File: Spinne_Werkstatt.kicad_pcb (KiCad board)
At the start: 2 copper layers, 15 parts, among them J1 Conn_01x02_Pin, J3 Conn_01x03_Pin, Q1 BSS138, Q2 BSS138, U2 CH340C, U4 ESP32-WROOM-32

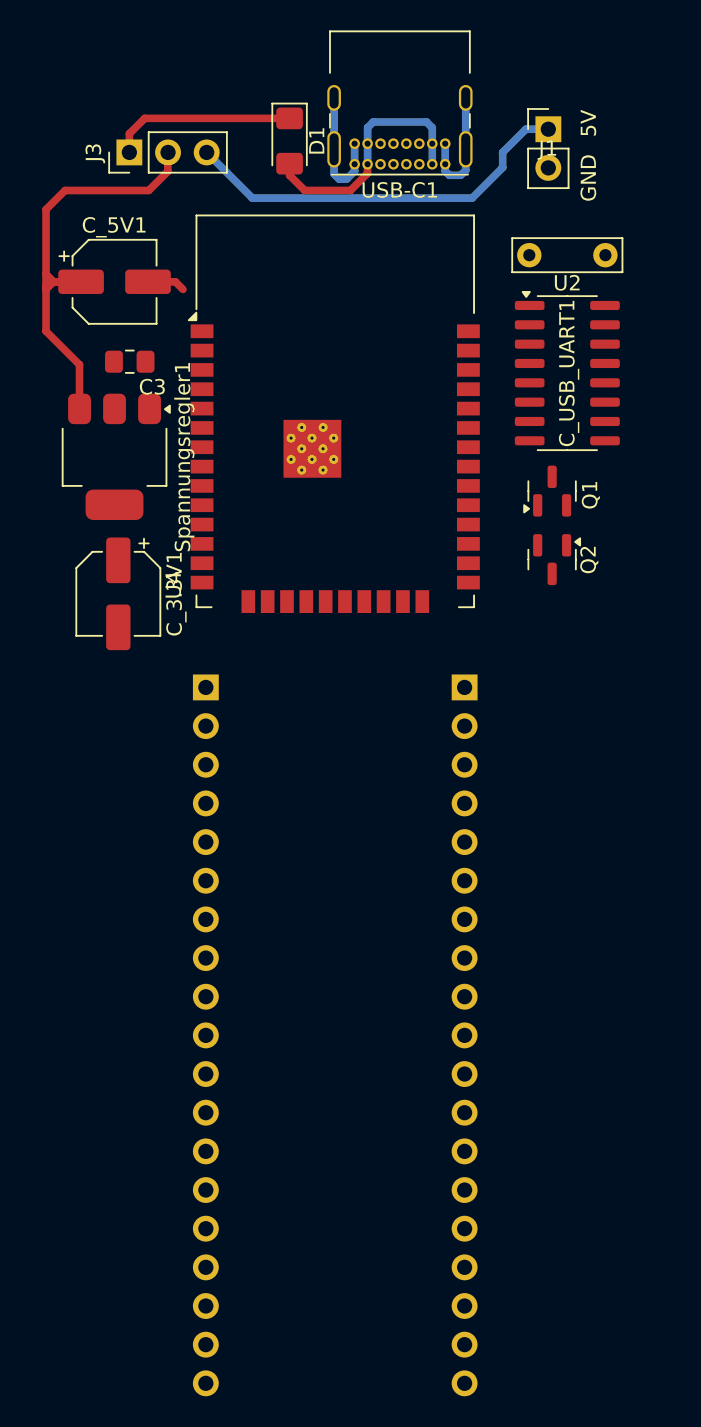
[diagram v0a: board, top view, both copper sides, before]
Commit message: finished first pcb -- ugly
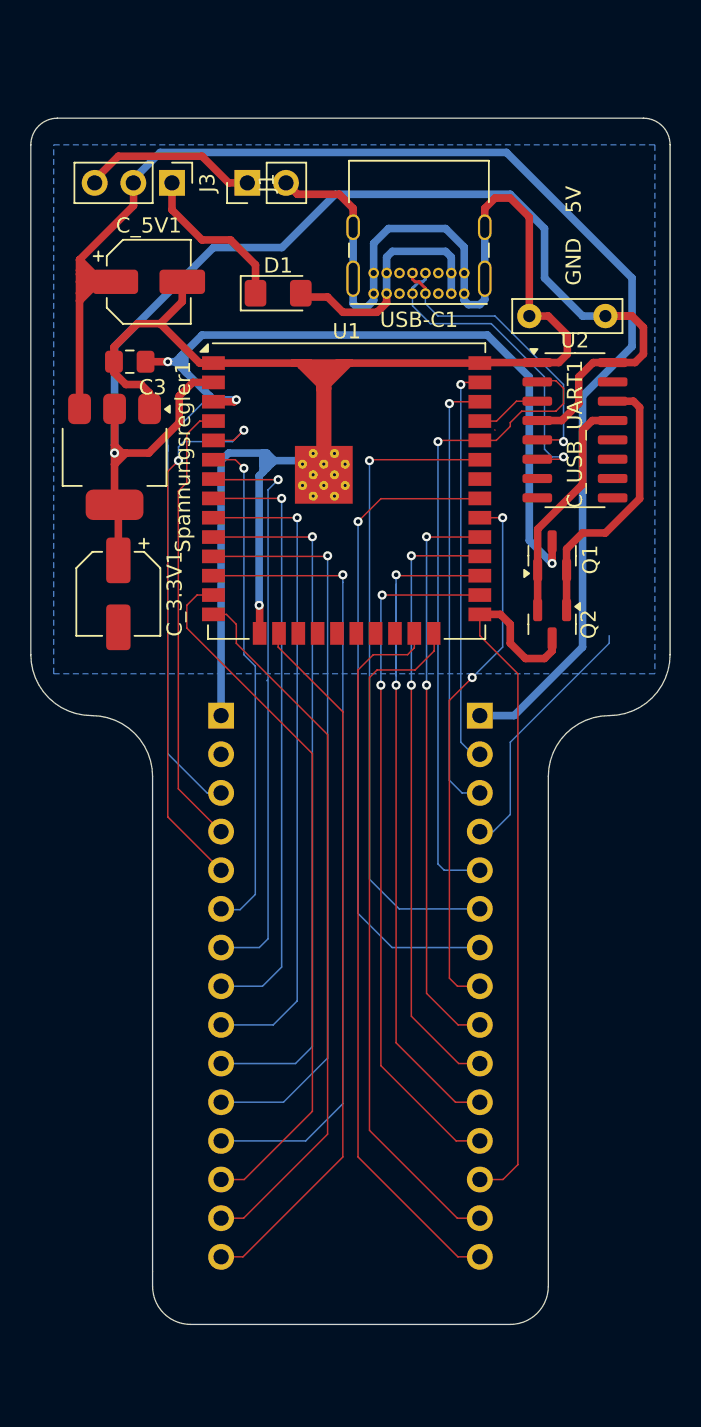
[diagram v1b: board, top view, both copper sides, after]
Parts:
- removed U4: ESP32-WROOM-32, bulme_footprints:ESP32-WROOM-32D
- added U1: ESP32-WROOM-32UE, RF_Module:ESP32-WROOM-32UE, F.Cu at (139.2, 62.8)
- esp_left1, esp_right1: value Conn_01x19_Pin -> Conn_01x15_Pin; footprint Connector_PinHeader_2.54mm:PinHeader_1x19_P2.54mm_Vertical -> Connector_PinHeader_2.54mm:PinHeader_1x15_P2.54mm_Vertical
- moved J1 20.1 mm to (132.7, 42.5), turned to 90 degrees
- moved D1 10.0 mm to (134.8, 49.8), turned to 0 degrees
- moved USB-C1 8.59 mm to (147.0, 49.8)
- moved Q1 4.25 mm to (152.8, 67.0)
- moved Q2 4.25 mm to (152.8, 71.5)
- moved C_USB_UART1 4.00 mm to (156.2, 51.2)
- moved U2 3.78 mm to (154.2, 58.8)
- moved J3 3.44 mm to (127.8, 42.5), turned to -90 degrees
- moved C_5V1 2.25 mm to (126.2, 49.0)
- moved esp_left1 2.10 mm to (131.0, 77.5)
- moved esp_right1 2.10 mm to (148.0, 77.5)
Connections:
- esp_left1 pad 15: pin15 -> pin16
- esp_right1 pad 10: pin29 -> pin28
- esp_right1 pad 11: pin28 -> pin27
- esp_right1 pad 12: pin27 -> pin26
- esp_right1 pad 13: pin26 -> ESP32_IO0
- esp_right1 pad 14: pin25 -> pin24
- esp_right1 pad 15: pin24 -> pin23
- esp_right1 pad 2: GND -> pin37
- esp_right1 pad 3: pin37 -> pin36
- esp_right1 pad 4: pin36 -> ESP32_TX
- esp_right1 pad 5: ESP32_TX -> ESP32_RX
- esp_right1 pad 6: ESP32_RX -> pin33
- esp_right1 pad 7: pin33 -> pin31
- esp_right1 pad 8: pin31 -> pin30
- esp_right1 pad 9: pin30 -> pin29
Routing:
- net GND: track 19.5 -> 164.2 mm, vias 0 -> 1
- net +3V3: track 0.00 -> 86.5 mm, vias 0 -> 1
- net ESP32_EN: track 0.00 -> 80.3 mm, vias 0 -> 3
- net +5V: track 30.1 -> 99.3 mm
- net pin12: track 0.00 -> 52.1 mm, vias 0 -> 1
- net pin27: track 0.00 -> 49.7 mm, vias 0 -> 2
- net pin23: track 0.00 -> 48.7 mm
- net pin11: track 0.00 -> 48.7 mm, vias 0 -> 1
- net ESP32_IO0: track 0.00 -> 47.8 mm
- net pin14: track 0.00 -> 47.0 mm
- net pin16: track 0.00 -> 46.9 mm
- net pin13: track 0.00 -> 46.6 mm
- net pin10: track 0.00 -> 46.5 mm, vias 0 -> 1
- net pin26: track 0.00 -> 46.0 mm, vias 0 -> 2
- net pin24: track 0.00 -> 45.6 mm
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- added copper zone on B.Cu, net GND
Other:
- board outline added: 42 x 79.2 mm

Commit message: nearly finished, not perfect but ok
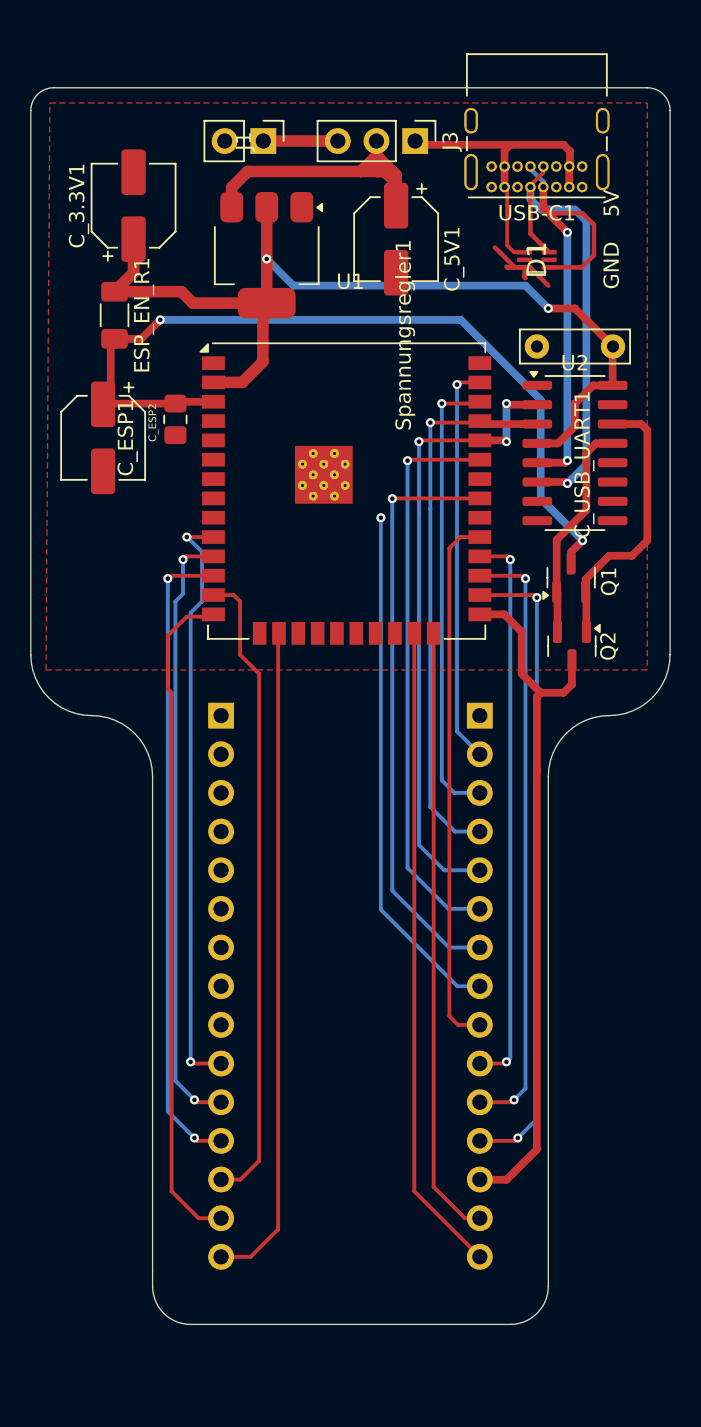
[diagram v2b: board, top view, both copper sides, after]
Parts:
- removed C3: 1uF, Capacitor_SMD:C_0805_2012Metric_Pad1.18x1.45mm_HandSolder
- added C_ESP1: 22uF, Capacitor_SMD:CP_Elec_5x5.7, F.Cu at (123.2, 59.2)
- added C_ESP2: 100nF, Capacitor_SMD:C_0805_2012Metric_Pad1.18x1.45mm_HandSolder, F.Cu at (128.0, 58.0)
- added ESP_EN_R1: 10k, Resistor_SMD:R_1206_3216Metric_Pad1.30x1.75mm_HandSolder, F.Cu at (124.0, 51.2)
- D1: value D_Schottky -> ESDAULC6-3BP6; footprint Diode_SMD:D_1206_3216Metric_Pad1.42x1.75mm_HandSolder -> bulme_footprints:ESDAULC63BP6
- moved C_3.3V1 25.5 mm to (125.2, 44.0), turned to 90 degrees
- moved D1 17.1 mm to (151.8, 47.6), turned to 90 degrees
- moved Spannungsregler1 16.6 mm to (134.0, 47.2)
- moved C_5V1 16.5 mm to (142.5, 46.2), turned to -90 degrees
- moved J3 16.2 mm to (143.8, 39.8)
- moved USB-C1 10.4 mm to (154.7, 42.8)
- moved J1 2.94 mm to (133.8, 39.8), turned to -90 degrees
- moved C_USB_UART1 2.06 mm to (156.8, 53.2)
- moved Q2 1.94 mm to (154.1, 72.9)
- moved Q1 1.90 mm to (154.0, 68.4)
- moved U2 1.50 mm to (154.2, 60.2)
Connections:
- net ESP32_RX renamed ESP_RX
- net ESP32_TX renamed ESP_TX
- D1 pad 1: VBUS -> D+
- D1 pad 2: Net-(D1-A) -> (no net)
- USB-C1 pad A4: Net-(D1-A) -> VBUS
- USB-C1 pad A9: Net-(D1-A) -> VBUS
- USB-C1 pad B4: Net-(D1-A) -> VBUS
- USB-C1 pad B9: Net-(D1-A) -> VBUS
- esp_left1 pad 2: +3.3V -> +3V3
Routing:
- net GND: track 164.2 -> 5.86 mm, vias 1 -> 0
- net +5V: track 99.3 -> 20.7 mm
- net pin9: track 42.9 -> 0.00 mm, vias 1 -> 0
- net pin8: track 39.8 -> 0.00 mm, vias 1 -> 0
- net pin7: track 38.4 -> 0.00 mm, vias 1 -> 0
- net pin5: track 36.6 -> 0.00 mm, vias 2 -> 0
- net pin6: track 33.3 -> 0.00 mm, vias 1 -> 0
- net pin4: track 29.6 -> 0.00 mm
- net ESP32_EN: track 80.3 -> 55.3 mm, vias 3 -> 2
- net +3V3: track 86.5 -> 63.4 mm, vias 1 -> 2
- net Net-(D1-A): track 16.5 -> 0.00 mm
- net ESP_TX: track 21.2 -> 36.3 mm, vias 0 -> 1
- net D+: track 20.0 -> 32.7 mm, vias 1 -> 2
- net VBUS: track 10.6 -> 21.2 mm
- net D-: track 21.3 -> 31.4 mm
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- added copper zone on F.Cu, net GND
- removed copper zone on B.Cu, net GND
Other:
- board size 42 x 79.2 mm -> 42 x 81.2 mm
